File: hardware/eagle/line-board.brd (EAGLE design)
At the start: 83.8 x 47.9 mm, 34 parts

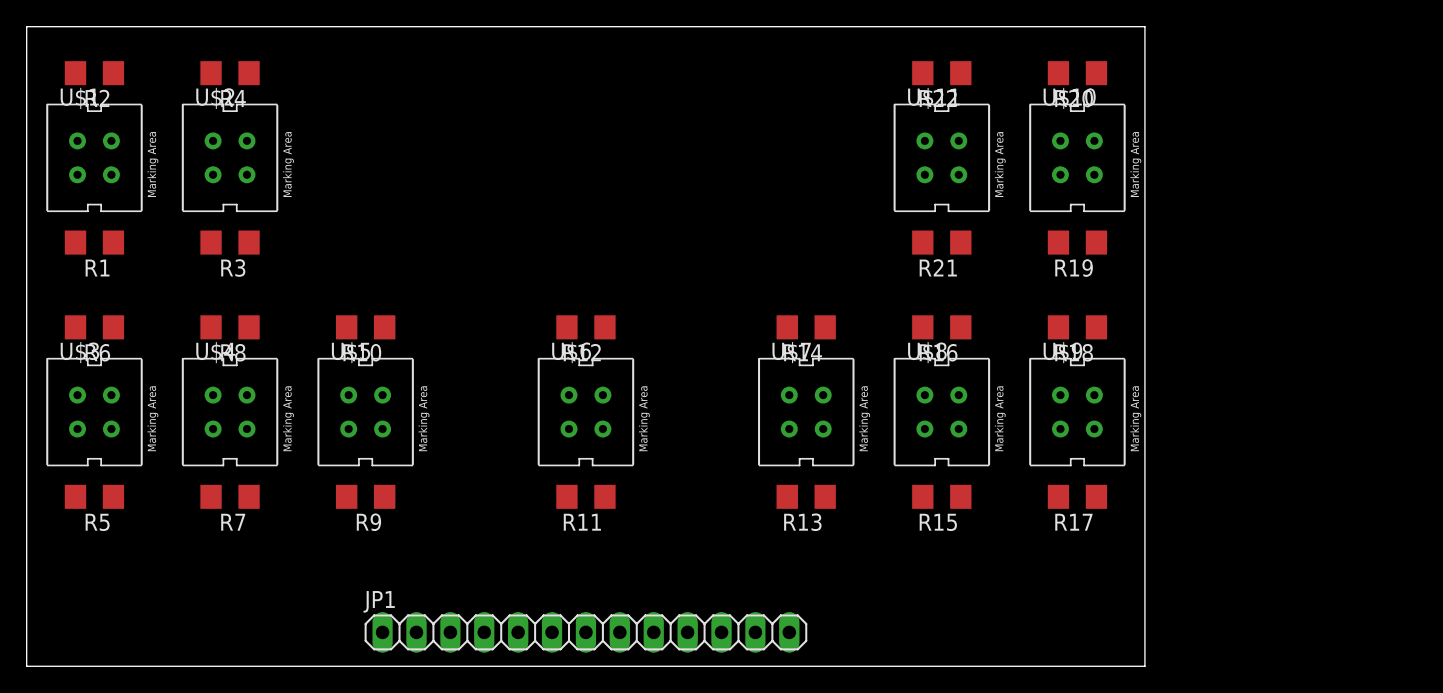
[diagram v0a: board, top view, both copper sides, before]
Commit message: layout
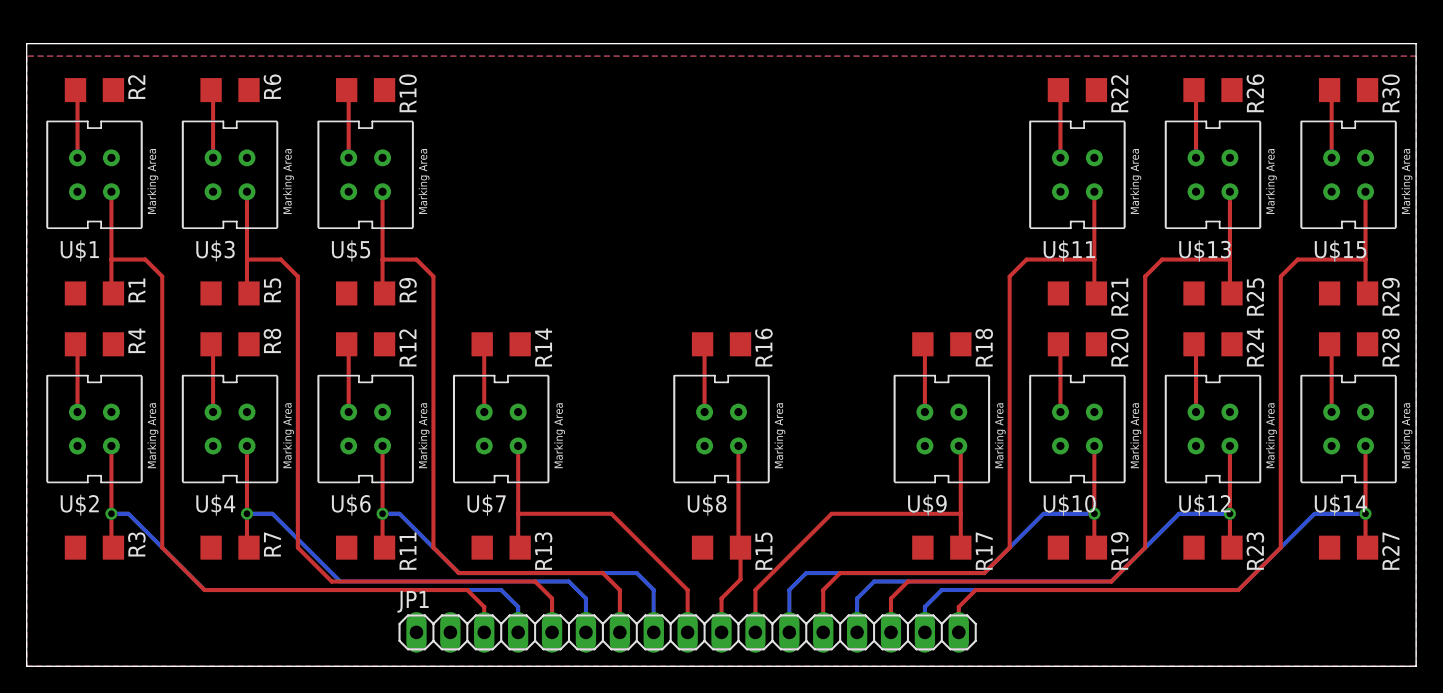
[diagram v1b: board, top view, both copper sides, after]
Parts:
- added R23, R25, R27, R29: 47k, rcl:R1206
- added R24, R26, R28, R30: 180, rcl:R1206
- added U$12, U$13, U$14, U$15: CNY70, cny70:4
- JP1: device pinhead:1X13 -> pinhead:1X17
- moved R3 25.0 mm to (5.08, 8.89)
- moved R13 23.2 mm to (35.6, 8.89)
- moved R14 22.9 mm to (35.6, 24.1)
- moved U$7 22.9 mm to (35.6, 17.8)
- moved R19 22.9 mm to (78.7, 8.89)
- moved R4 22.7 mm to (5.08, 24.1)
- moved U$2 22.7 mm to (5.08, 17.8)
- moved R6 20.5 mm to (15.2, 43.2)
- moved U$3 20.5 mm to (15.2, 36.8)
- moved R20 20.3 mm to (78.7, 24.1)
- moved U$10 20.3 mm to (78.7, 17.8)
- moved R5 18.3 mm to (15.2, 27.9)
- moved R10 17.8 mm to (25.4, 43.2)
- moved U$5 17.8 mm to (25.4, 36.8)
- moved R11 16.9 mm to (25.4, 8.89)
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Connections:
- new net N$1: R24.2, U$12.A
- new net N$4: R26.2, U$13.A
- new net N$6: R28.2, U$14.A
- new net N$8: R30.2, U$15.A
- new net S12: JP1.14, R23.1, U$12.C
- new net S13: JP1.15, R25.1, U$13.C
- new net S14: JP1.16, R27.1, U$14.C
- new net S15: JP1.17, R29.1, U$15.C
- net +5V: now also R23.2, R24.1, R25.2, R26.1, R27.2, R28.1, R29.2, R30.1
- net GND: now also U$12.E, U$12.K, U$13.E, U$13.K, U$14.E, U$14.K, U$15.E, U$15.K
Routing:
- net S15: track 0.00 -> 62.8 mm
- net S1: track 0.00 -> 60.2 mm
- net S13: track 0.00 -> 58.0 mm
- net S3: track 0.00 -> 55.5 mm
- net S11: track 0.00 -> 53.3 mm
- net S5: track 0.00 -> 50.8 mm
- net S14: track 0.00 -> 45.5 mm, vias 0 -> 1
- net S2: track 0.00 -> 43.0 mm, vias 0 -> 1
- net S12: track 0.00 -> 40.8 mm, vias 0 -> 1
- net S4: track 0.00 -> 38.3 mm, vias 0 -> 1
- net S10: track 0.00 -> 36.1 mm, vias 0 -> 1
- net S6: track 0.00 -> 33.5 mm, vias 0 -> 1
- net S9: track 0.00 -> 28.8 mm
- net S7: track 0.00 -> 25.9 mm
- net S8: track 0.00 -> 14.6 mm
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- added copper zone on layer 1, net +5V
- added copper zone on layer 16, net GND
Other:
- board size 83.8 x 47.9 mm -> 104.1 x 46.7 mm
